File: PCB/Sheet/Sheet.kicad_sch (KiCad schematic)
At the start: 2 parts, among them U1 74LVC2G74, U2 SN74LVC1G00DBV

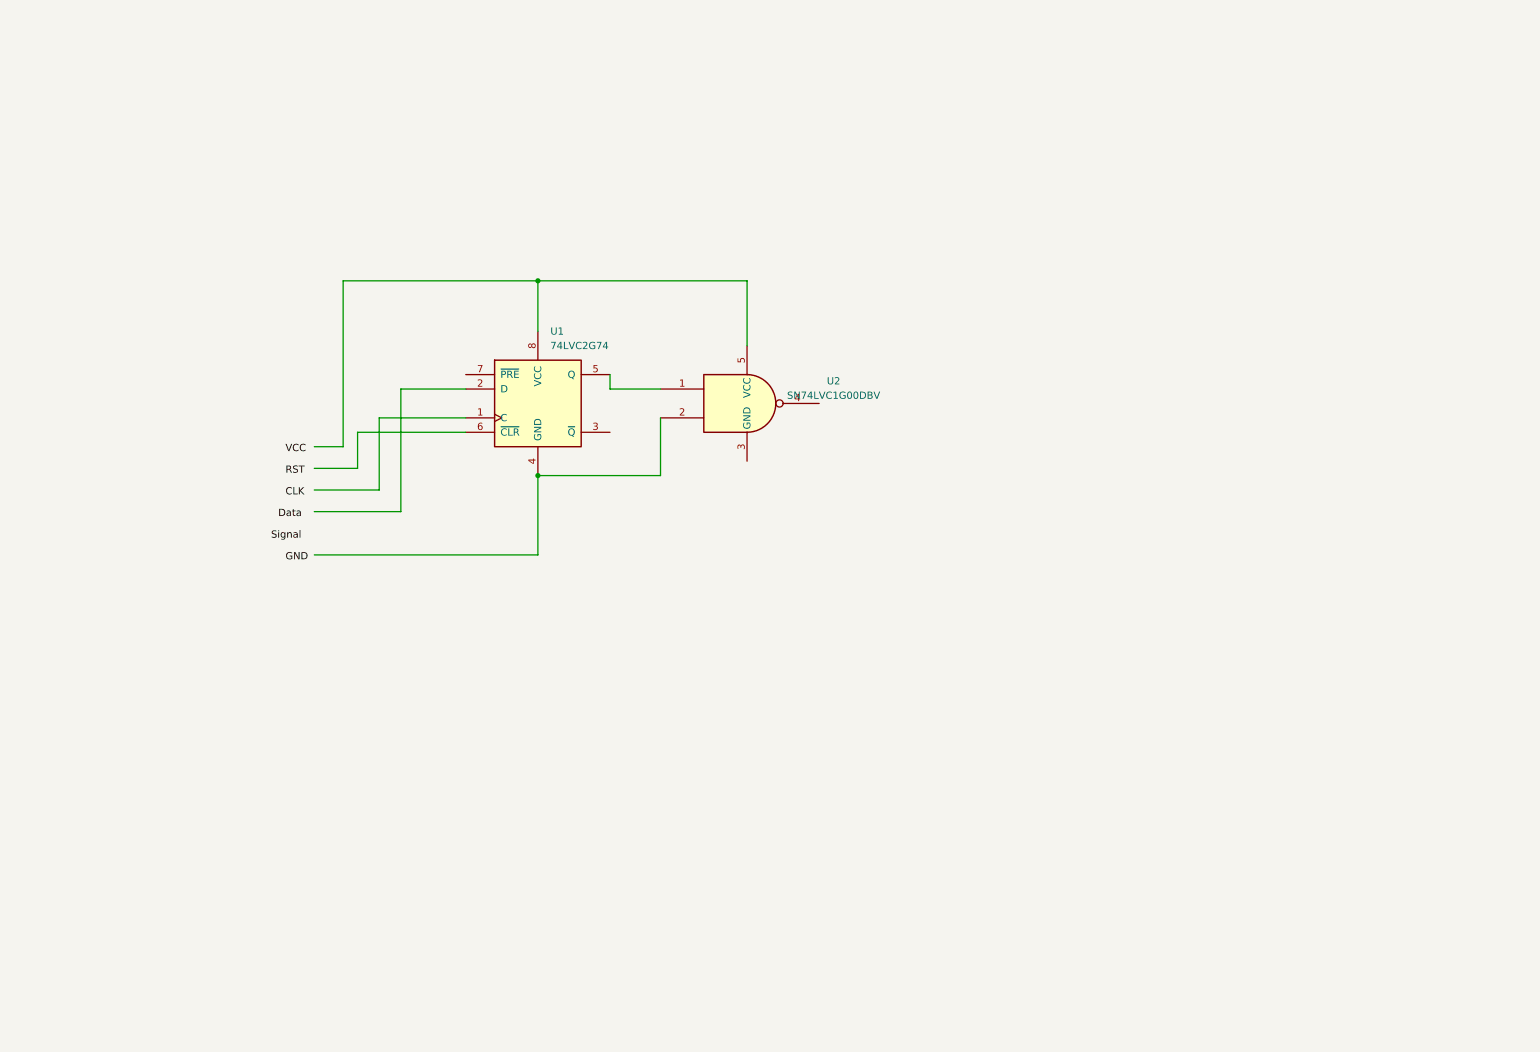
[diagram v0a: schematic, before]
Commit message: Update Sheet.kicad_sch
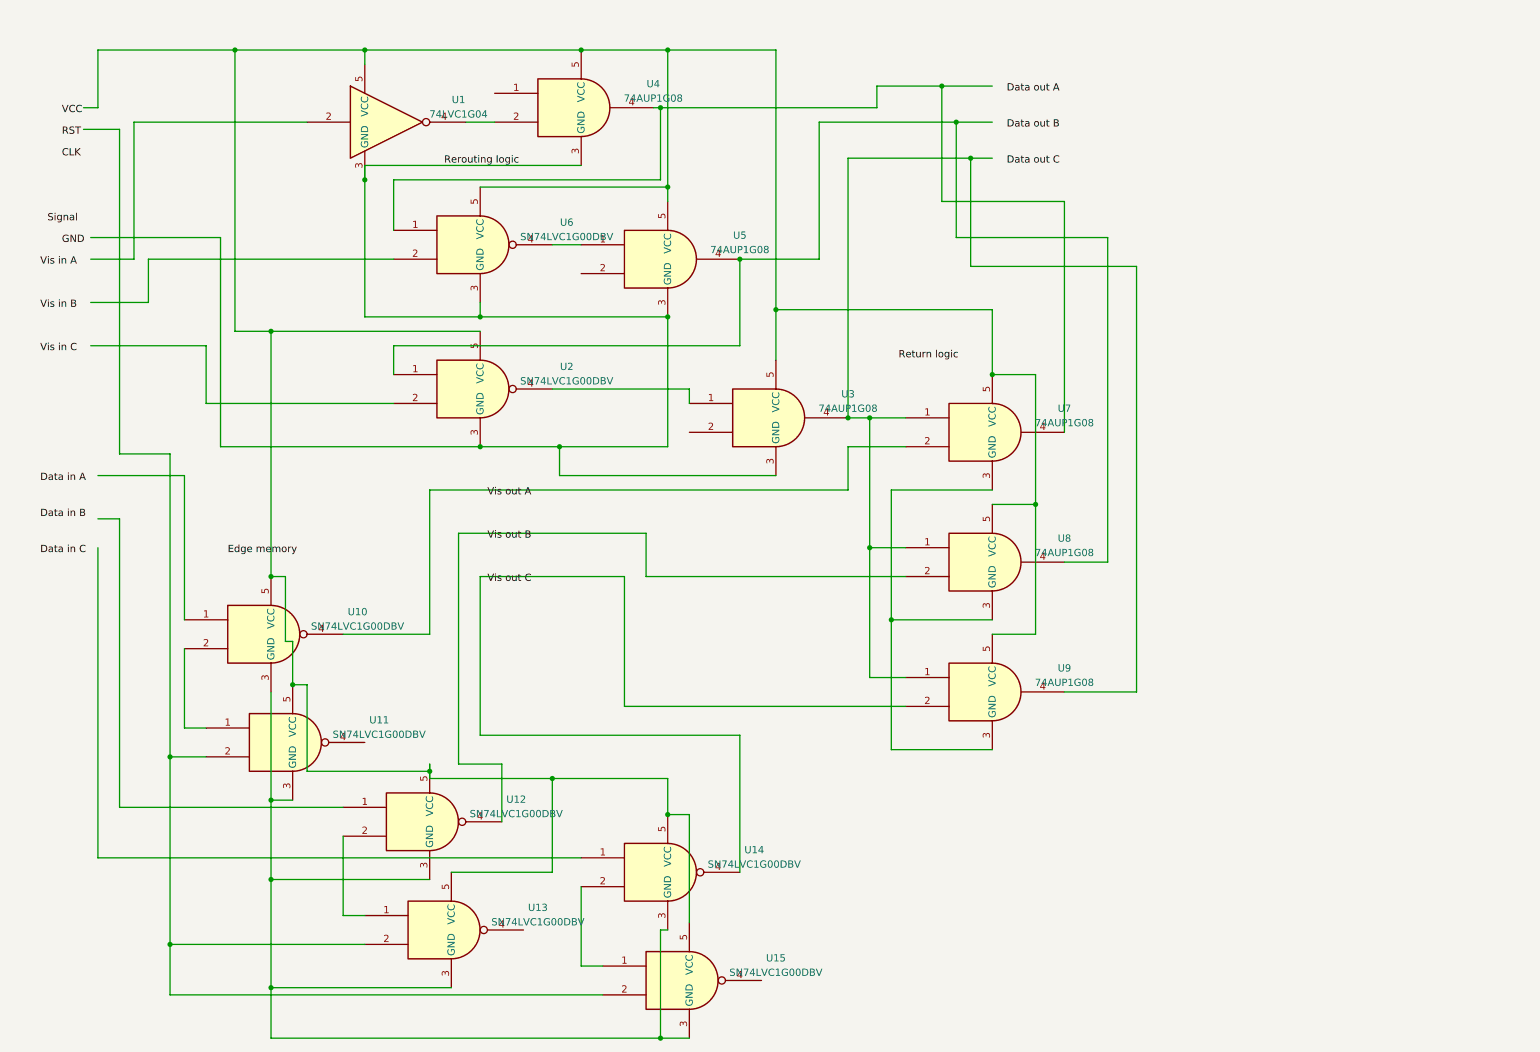
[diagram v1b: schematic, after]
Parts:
- removed U1: 74LVC2G74, symbol 74xGxx:74LVC2G74
- added U1: 74LVC1G04, symbol 74xGxx:74LVC1G04
- added U10, U11, U12, U13, U14, U15, U6: SN74LVC1G00DBV, Package_TO_SOT_SMD:SOT-23-5, symbol 74xGxx:SN74LVC1G00DBV
- added U3, U4, U5, U7, U8, U9: 74AUP1G08, symbol 74xGxx:74AUP1G08
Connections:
- net at U2.1: now also U5.4, U8.4
- net Rerouting logic: now reaches U2.3 (GND)
- net Rerouting logic: now also U1.3 (GND), U3.3 (GND), U4.3 (GND), U5.3 (GND), U6.3 (GND)
- net at U2.4: now also U3.1
- net at U2.5 (VCC): now also U1.5 (VCC), U10.5 (VCC), U11.5 (VCC), U12.5 (VCC), U13.5 (VCC), U14.5 (VCC), U15.5 (VCC), U3.5 (VCC), U4.5 (VCC), U5.5 (VCC), U6.5 (VCC), U7.5 (VCC), U8.5 (VCC), U9.5 (VCC)
- new net: U3.4, U7.1, U8.1, U9.1, U9.4
- new net: U10.4, U7.2
- new net: U7.3 (GND), U8.3 (GND), U9.3 (GND)
- new net: U4.4, U6.1, U7.4
- new net: U10.2, U11.1
- new net: U10.3 (GND), U11.3 (GND), U12.3 (GND), U13.3 (GND), U14.3 (GND), U15.3 (GND)
- new net: U14.2, U15.1
- new net: U14.4, U9.2
- new net: U11.2, U13.2, U15.2
- new net: U5.1, U6.4
- new net: U12.2, U13.1
- new net: U12.4, U8.2
- new net: U1.4, U4.2
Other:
- company: (none) -> Dexter R. Shepherd
- title: (none) -> TacSheet flexible sensor

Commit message: Update Sheet.kicad_sch
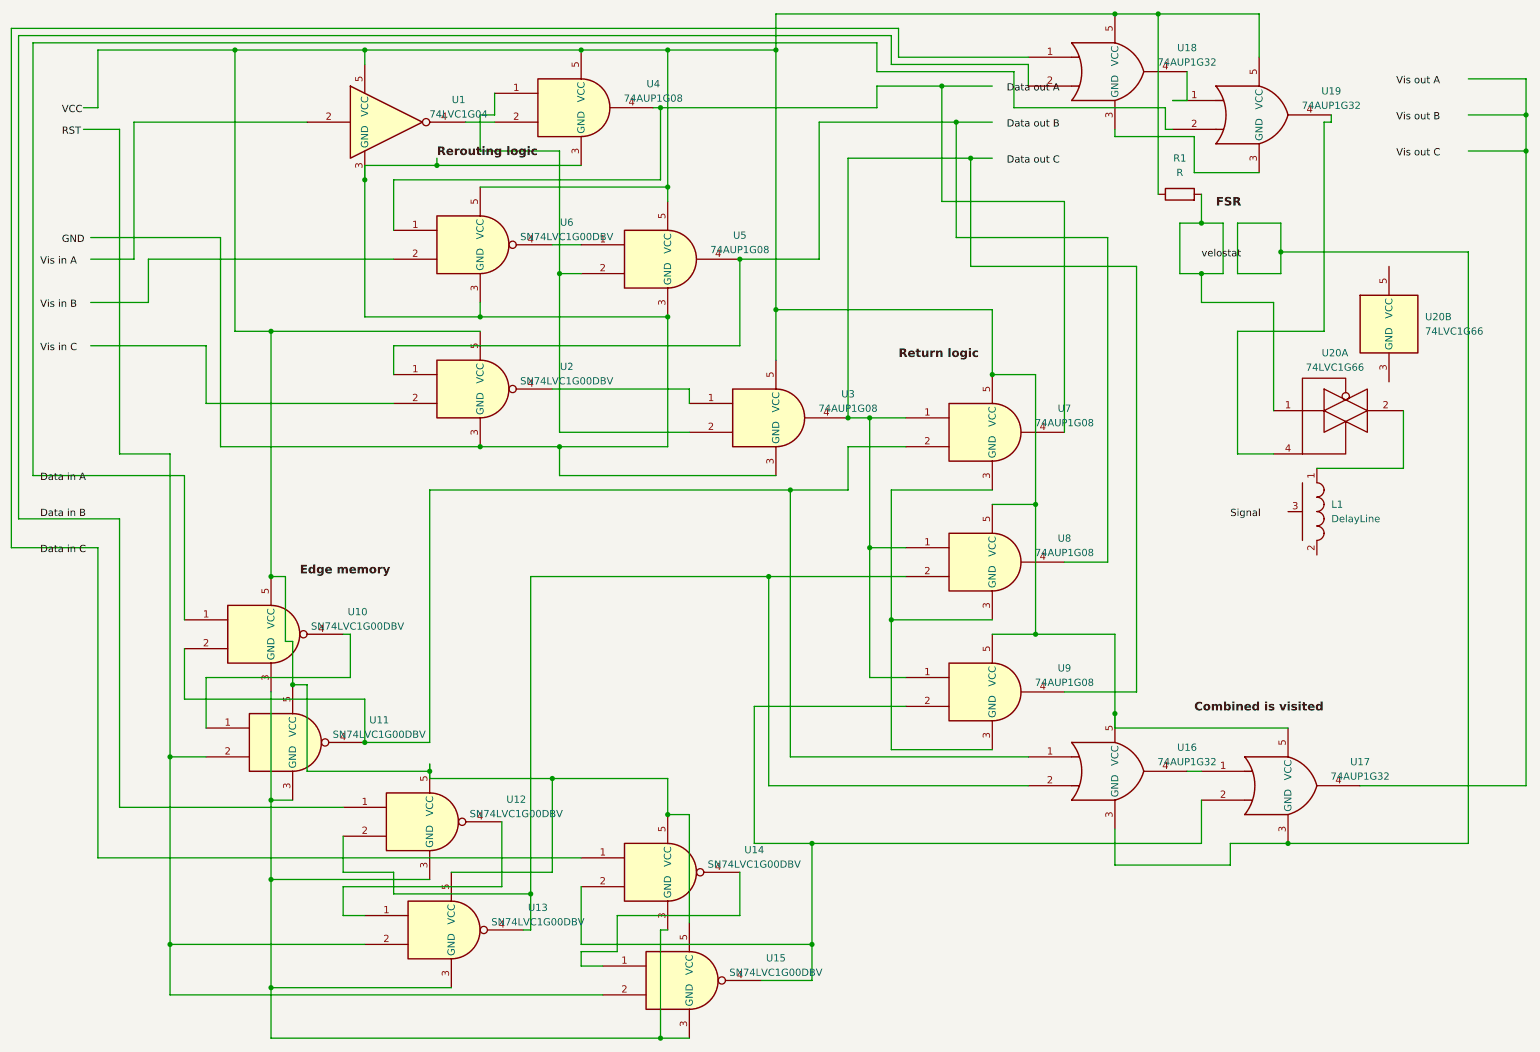
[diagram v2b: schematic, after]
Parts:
- added L1: DelayLine, symbol Device:DelayLine
- added R1: R, symbol Device:R
- added U16, U17, U18, U19: 74AUP1G32, symbol 74xGxx:74AUP1G32
- added U20: 74LVC1G66, symbol 74xGxx:74LVC1G66
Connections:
- net Data in B: now also U12.1, U18.2
- net at U7.2: now also U10.2, U11.4, U16.1; no longer U10.4
- net at U1.5 (VCC), U10.5 (VCC), U11.5 (VCC)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: now also R1.1, U16.5 (VCC), U17.5 (VCC), U18.5 (VCC), U19.5 (VCC)
- net at U10.1: now also U19.2
- net at U11.1: now also U10.4; no longer U10.2
- net at U14.1: now also U18.1
- net at U14.2: now also U15.4, U9.2, U17.2; no longer U15.1
- net at U14.4: now also U15.1; no longer U9.2
- net at U5.2: now also U3.2, U4.1
- net at U12.2: now also U13.4, U8.2, U16.2; no longer U13.1
- net at U12.4: now also U13.1; no longer U8.2
- new net: L1.1, U20.2
- new net: R1.2, U20.1
- new net: U19.4, U20.4
- new net: U16.3 (GND), U17.3 (GND)
- new net: U16.4, U17.1
- new net: U18.4, U19.1
- new net: U18.3 (GND), U19.3 (GND)

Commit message: schematics
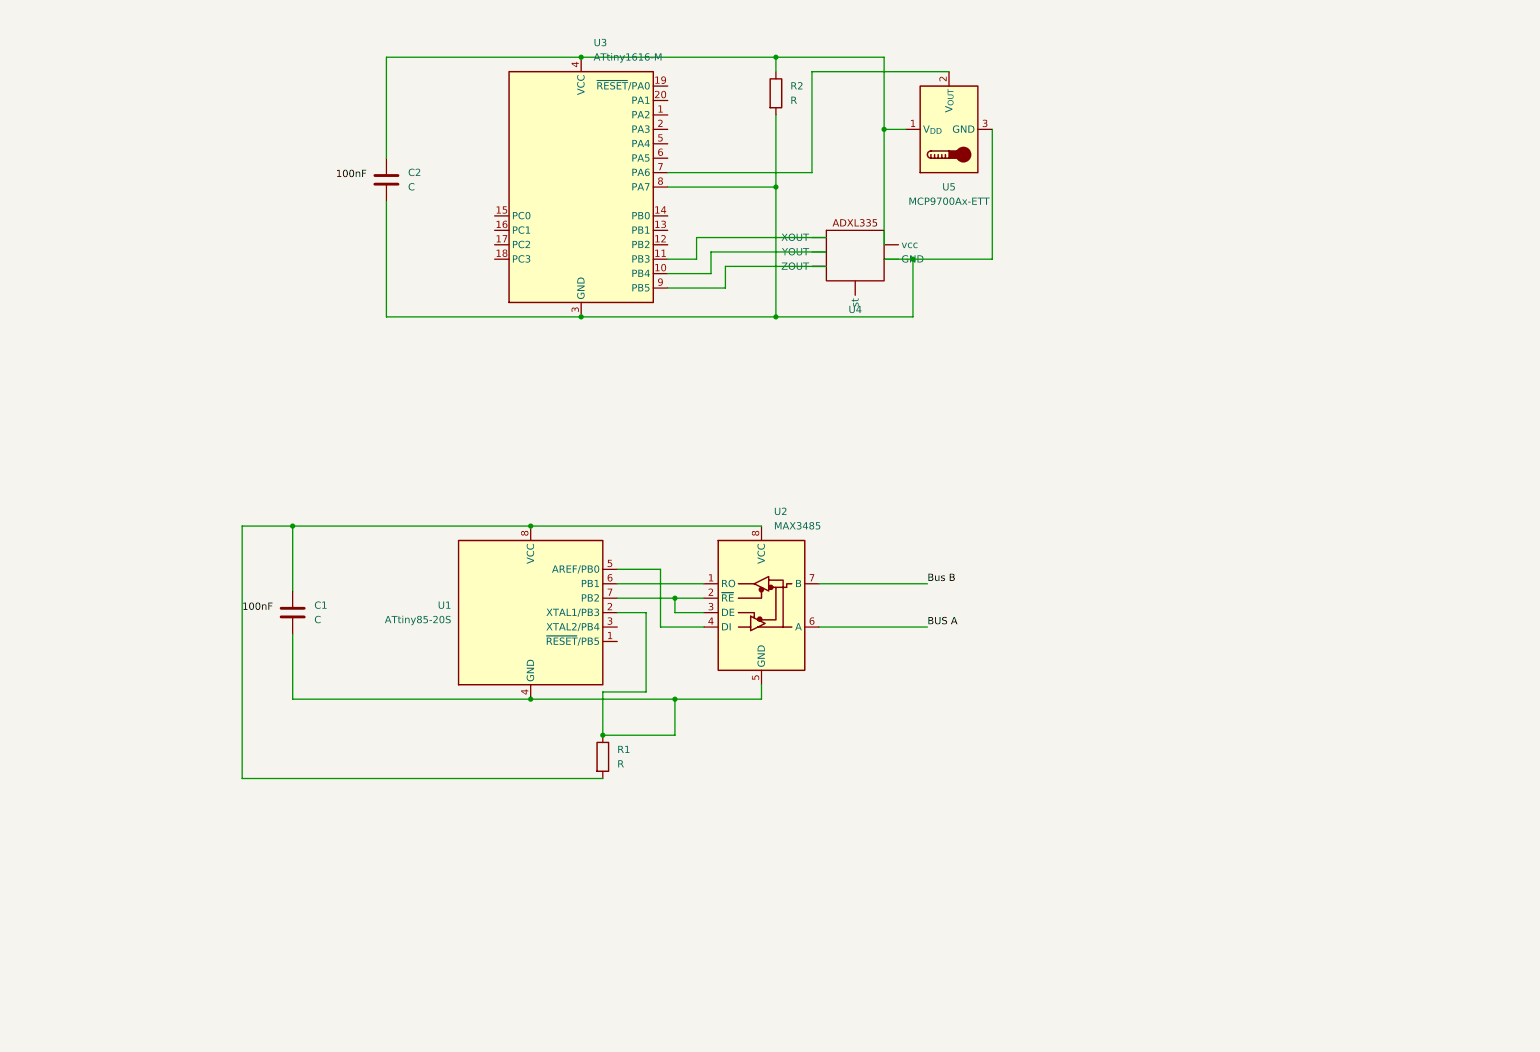
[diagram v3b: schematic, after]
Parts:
- removed L1: DelayLine, symbol Device:DelayLine
- removed U1: 74LVC1G04, symbol 74xGxx:74LVC1G04
- removed U10, U11, U12, U13, U14, U15, U2, U6: SN74LVC1G00DBV, Package_TO_SOT_SMD:SOT-23-5, symbol 74xGxx:SN74LVC1G00DBV
- removed U16, U17, U18, U19: 74AUP1G32, symbol 74xGxx:74AUP1G32
- removed U20: 74LVC1G66, symbol 74xGxx:74LVC1G66
- removed U3, U4, U5, U7, U8, U9: 74AUP1G08, symbol 74xGxx:74AUP1G08
- added C1, C2: C, symbol Device:C
- added R2: R, symbol Device:R
- added U1: ATtiny85-20S, Package_SO:SOIC-8W_5.3x5.3mm_P1.27mm, symbol MCU_Microchip_ATtiny:ATtiny85-20S
- added U2: MAX3485, symbol Interface_UART:MAX3485
- added U3: ATtiny1616-M, Package_DFN_QFN:VQFN-20-1EP_3x3mm_P0.4mm_EP1.7x1.7mm, symbol MCU_Microchip_ATtiny:ATtiny1616-M
- added U4: ~, symbol sensors:ADXL335
- added U5: MCP9700Ax-ETT, Package_TO_SOT_SMD:SOT-23, symbol Sensor_Temperature:MCP9700Ax-ETT
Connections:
- net at R1.1: now also C1.2, U1.2 (XTAL1/PB3), U1.4 (GND), U2.5 (GND)
- net 100nF: now reaches R1.2
- net 100nF: now also C1.1, U1.8 (VCC), U2.8 (VCC)
- new net: U1.5 (AREF/PB0), U2.4 (DI)
- new net: U1.6 (PB1), U2.1 (RO)
- new net: U1.7 (PB2), U2.2 (~{RE}), U2.3 (DE)
- new net: U3.10 (PB4), U4. (vcc)
- new net: U3.11 (PB3), U4. (vcc)
- new net: C2.2, R2.2, U3.21 (GND), U3.3 (GND), U3.8 (PA7), U4. (vcc), U5.3 (GND)
- new net: C2.1, R2.1, U3.4 (VCC), U4. (vcc), U5.1 (V_{DD})
- new net: U3.7 (PA6), U5.2 (V_{OUT})
- new net: U3.9 (PB5), U4. (vcc)
- new net BUS A: U2.6 (A)
- new net Bus B: U2.7 (B)
